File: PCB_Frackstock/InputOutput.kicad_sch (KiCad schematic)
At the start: 30 parts, among them J1 Conn_01x06_Pin, U11 CC1101RGPR, U7 BMI323, Y2 26MHz

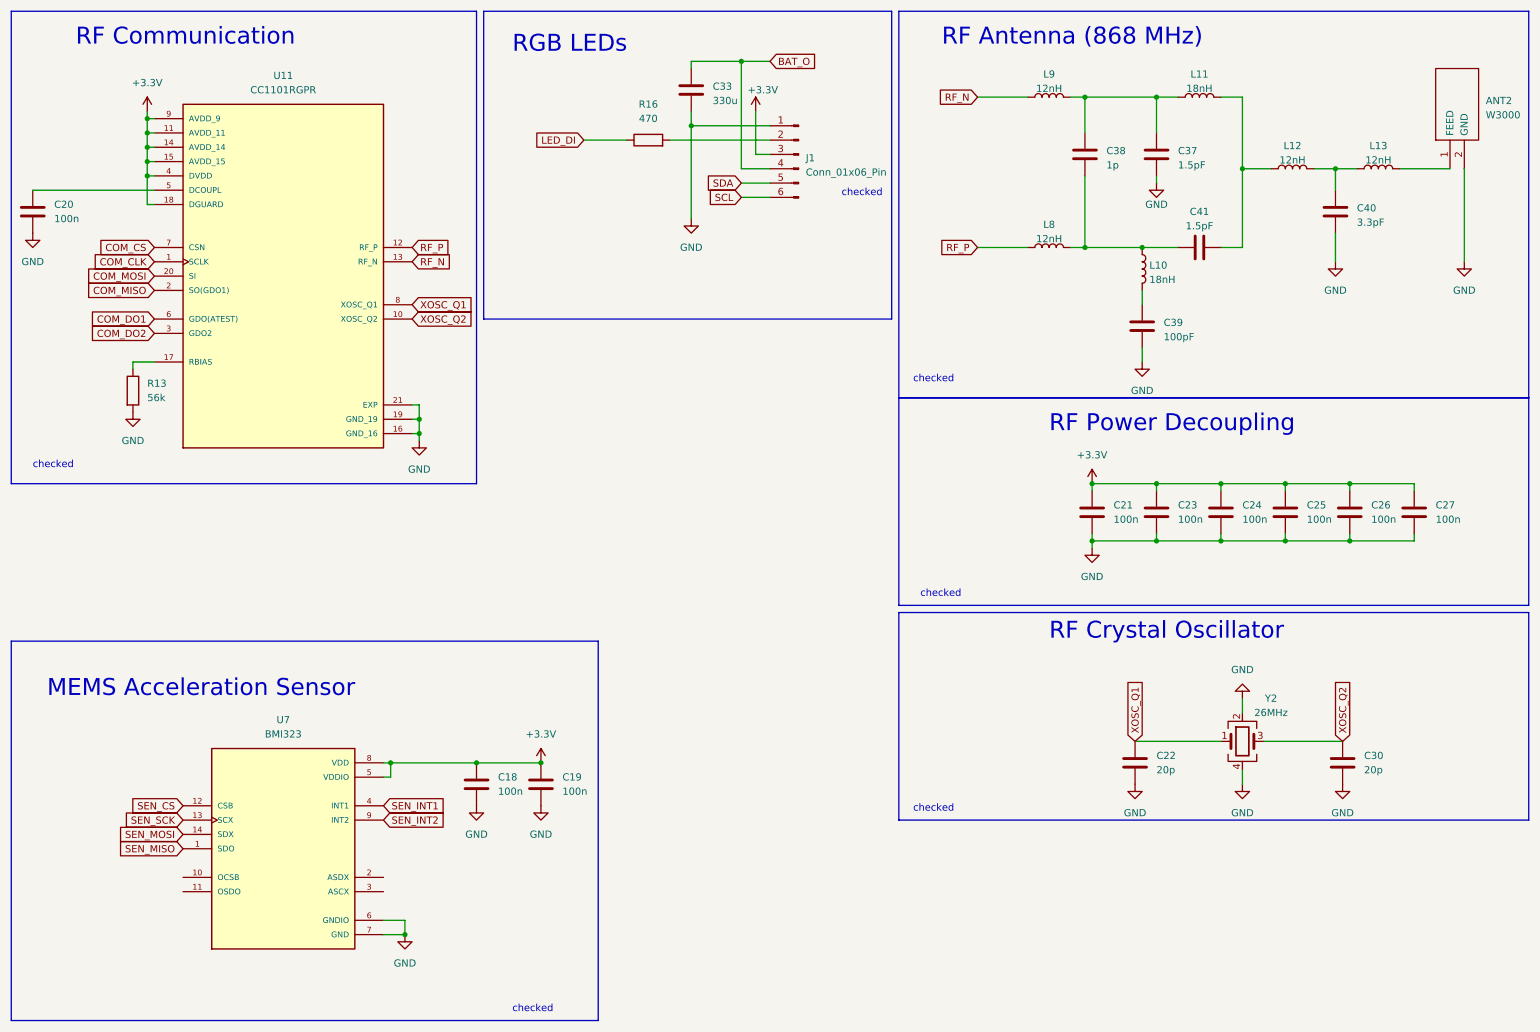
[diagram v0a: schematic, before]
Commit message: Schema-review-1
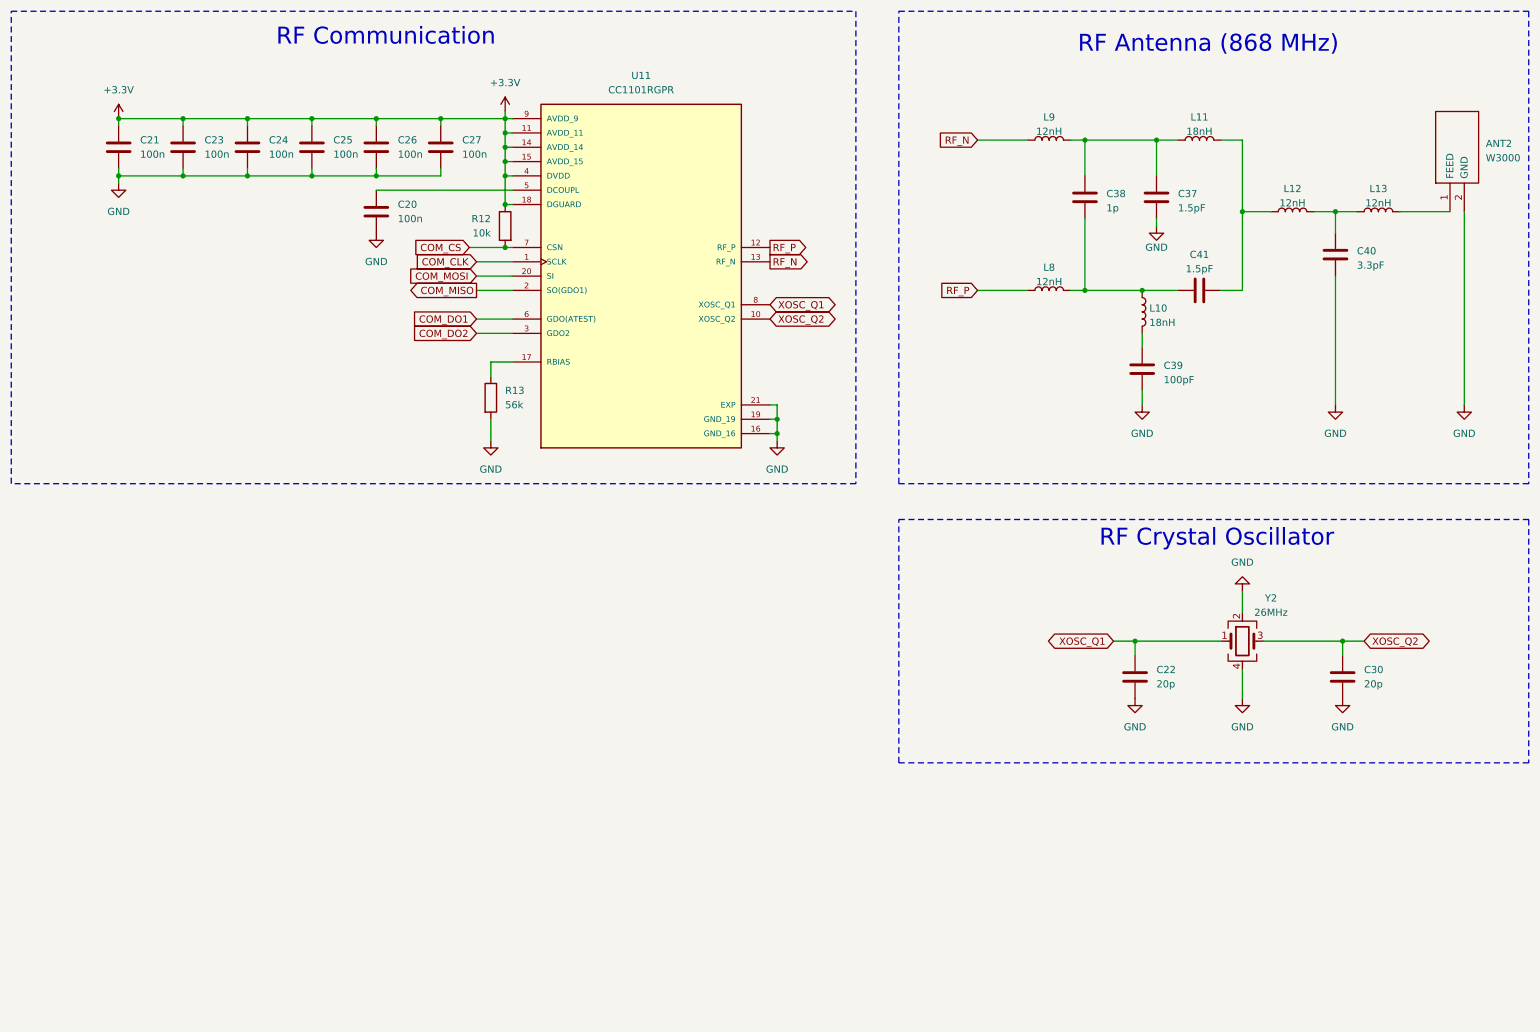
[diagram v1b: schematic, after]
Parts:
- removed C18, C19: 100n, Capacitor_SMD:C_0603_1608Metric_Pad1.08x0.95mm_HandSolder, symbol Device:C
- removed C33: 330u, Capacitor_SMD:C_0805_2012Metric_Pad1.18x1.45mm_HandSolder, symbol Device:C
- removed J1: Conn_01x06_Pin, Frack:PinHeader_2x03_P2.54mm_Vertical_SMD_kleiner, symbol Connector:Conn_01x06_Pin
- removed R16: 470, Resistor_SMD:R_0603_1608Metric_Pad0.98x0.95mm_HandSolder, symbol Device:R
- removed U7: BMI323, SnapEDA Library:PQFN50P250X300X88-14N, symbol BMI160:BMI160
- added R12: 10k, Resistor_SMD:R_0603_1608Metric_Pad0.98x0.95mm_HandSolder, symbol Device:R
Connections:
- net +3.3V: now also R12.1
- net COM_CS: now also R12.2
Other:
- note removed: "MEMS Acceleration Sensor"
- note removed: "RF Power Decoupling"
- note removed: "RGB LEDs"
- note removed: "checked"
- company: (none) -> Eberkreis
- title: (none) -> Frackstock ET2024
- moved on the sheet: ANT2, C20, C21, C22, C23, C24, C25, C26, C27, C30, C37, C38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
